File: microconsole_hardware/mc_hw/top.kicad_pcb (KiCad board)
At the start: 2 copper layers, 161 x 96 mm, 115 parts, among them J2 USB_C_Receptacle, Q1 DMP2035U-7, Q2 DMP2035U-7, SW10 TL3301NF160QG, SW11 TL3301NF160QG, SW12 TL3301NF160QG, SW13 TL3301NF160QG, SW14 TL3301NF160QG, SW15 TL3301NF160QG, SW16 Joystick, SW17 Joystick, SW19 SPDT_Slide_PTH_11.6x4.0mm, SW2 TL3301NF160QG, SW3 TL3301NF160QG, SW4 TL3301NF160QG, SW5 TL3301NF160QG, SW6 TL3301NF160QG, SW7 TL3301NF160QG, SW8 TL3301NF160QG, SW9 TL3301NF160QG, U1 MCP73833-FCI/UN, U2 S2B-PH-K-S, U3 MCP23017-E/SO, U4 ADS7828E/2K5, U5 PCM5102APWR, U6 PAM8302AADCR, U7 PAM8406DR

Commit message: fix2
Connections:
- U1 pad 1: unconnected-(U1-VDD-Pad1) -> USB-VBUS
- U1 pad 10: unconnected-(U1-V_{BAT}-Pad10) -> BAT+
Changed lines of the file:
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@@
 			)
 		)
-		(property ki_fp_filters "R_* RV_*")
+		(property ki_fp_filters "PinHeader_1x02_P2.54mm_*")
 		(sheetname "/Battery/")
 		(sheetfile "battery.kicad_sch")
@@
 		)
 		(embedded_fonts no)
-		(model "${KICAD8_3DMODEL_DIR}/Capacitor_SMD.3dshapes/C_0805_2012Metric.wrl"
+		(model "${KICAD10_3DMODEL_DIR}/Capacitor_SMD.3dshapes/C_0805_2012Metric.step"
 			(offset
 				(xyz 0 0 0)
@@
 		)
 		(embedded_fonts no)
-		(model "${KICAD8_3DMODEL_DIR}/Capacitor_SMD.3dshapes/C_0805_2012Metric.wrl"
+		(model "${KICAD10_3DMODEL_DIR}/Capacitor_SMD.3dshapes/C_0805_2012Metric.step"
 			(offset
 				(xyz 0 0 0)
@@
 			)
 		)
-		(property ki_fp_filters "SOT?23*")
+		(property ki_fp_filters "MSOP-10*")
 		(sheetname "/Battery/")
 		(sheetfile "battery.kicad_sch")
@@
 			(unit
 				(name "A")
-				(pins "9" "8" "6" "1" "5" "10" "2" "3" "4" "7")
+				(pins "9" "8" "6" "10" "5" "1" "2" "3" "4" "7")
 			)
 		)
@@
 			(size 0.3 1)
 			(layers "B.Cu")
-			(net "unconnected-(U1-VDD-Pad1)")
+			(net "USB-VBUS")
 			(pinfunction "VDD_1")
-			(pintype "power_in+no_connect")
+			(pintype "power_in")
 			(thermal_bridge_angle 0)
 		)
@@
 			(size 0.3 1)
 			(layers "B.Cu")
-			(net "unconnected-(U1-V_{BAT}-Pad10)")
+			(net "BAT+")
 			(pinfunction "V_{BAT}_10")
-			(pintype "power_out+no_connect")
+			(pintype "power_out")
 			(thermal_bridge_angle 0)
 		)
@@
 			)
 		)
-		(property "Datasheet" ""
+		(property "Datasheet" "https://assets.nexperia.com/documents/data-sheet/PMEG40T30ER.pdf"
 			(at 0 0 270)
 			(unlocked yes)
@@
 			)
 		)
-		(attr smd)
+		(attr smd dnp)
 		(duplicate_pad_numbers_are_jumpers no)
 		(fp_line

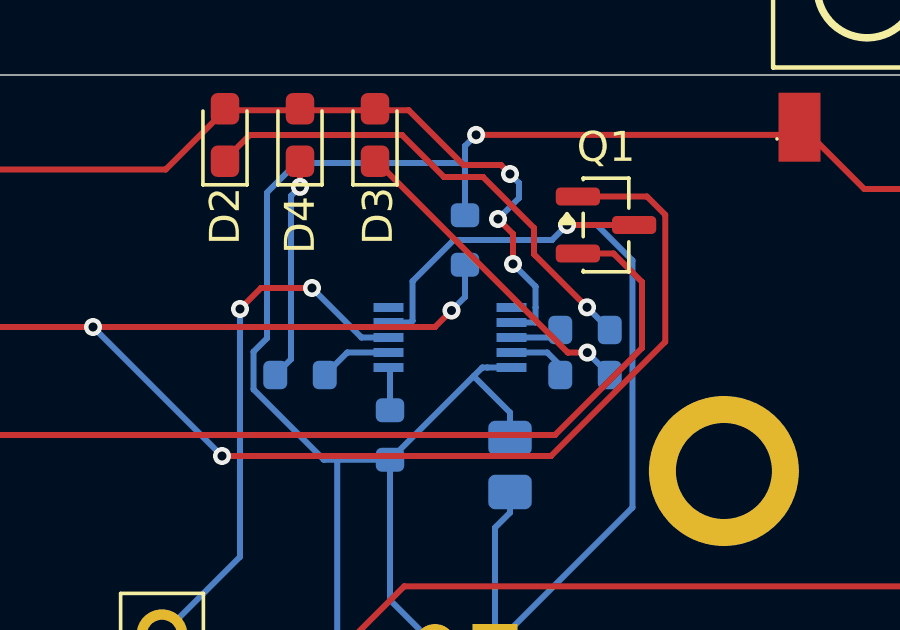
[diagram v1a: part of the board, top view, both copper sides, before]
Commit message: fix up
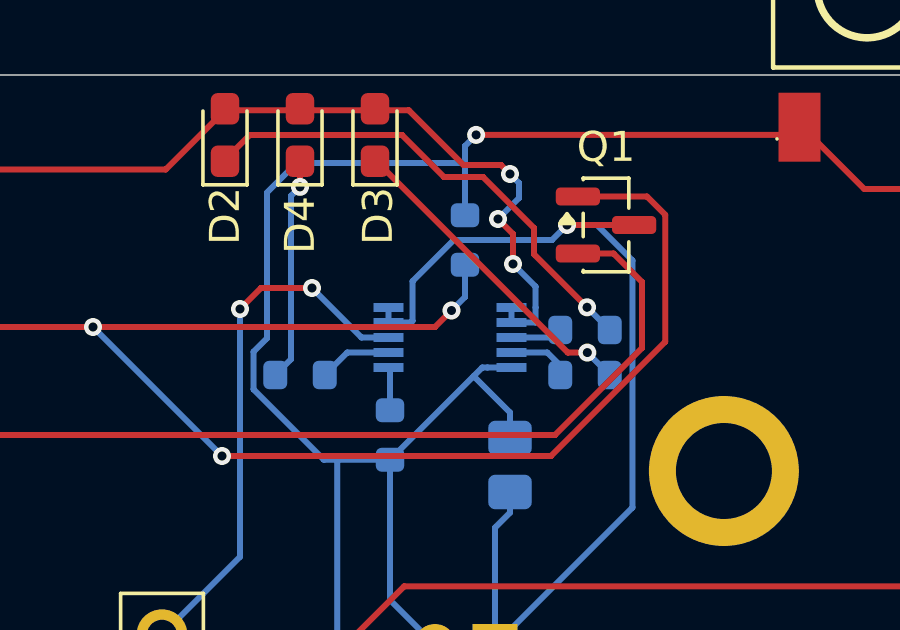
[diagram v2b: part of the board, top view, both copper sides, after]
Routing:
- net USB-VBUS: track 91.6 -> 92.1 mm
- net BAT+: track 32.6 -> 33.1 mm
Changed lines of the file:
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@@
 			(net "USB-VBUS")
 			(pinfunction "VDD_1")
-			(pintype "power_in")
+			(pintype "passive")
 			(thermal_bridge_angle 0)
 		)
@@
 			(net "BAT+")
 			(pinfunction "V_{BAT}_10")
-			(pintype "power_out")
+			(pintype "passive")
 			(thermal_bridge_angle 0)
 		)
@@
 			)
 		)
-		(property ki_fp_filters "TO-???* *_Diode_* *SingleDiode* D_*")
+		(property ki_fp_filters "TO-???* *_Diode_* *SingleDiode* D_* Diode_*")
 		(sheetname "/Battery/")
 		(sheetfile "battery.kicad_sch")
@@
 			)
 		)
-		(attr smd dnp)
+		(attr smd)
 		(duplicate_pad_numbers_are_jumpers no)
 		(fp_line
@@
 	)
 	(segment
+		(start 190.55 65.75)
+		(end 190.55 66.25)
+		(width 0.2)
+		(layer "B.Cu")
+		(net "USB-VBUS")
+	)
+	(segment
 		(start 191.3517 65.75)
 		(end 191.3517 65.0517)
@@
 		(width 0.2)
 		(layer "B.Cu")
+		(net "BAT+")
+	)
+	(segment
+		(start 186.45 65.75)
+		(end 186.45 66.25)
+		(width 0.2)
+		(layer "B.Cu")
